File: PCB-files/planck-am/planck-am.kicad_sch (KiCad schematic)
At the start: 97 parts, among them U1 ProMicro

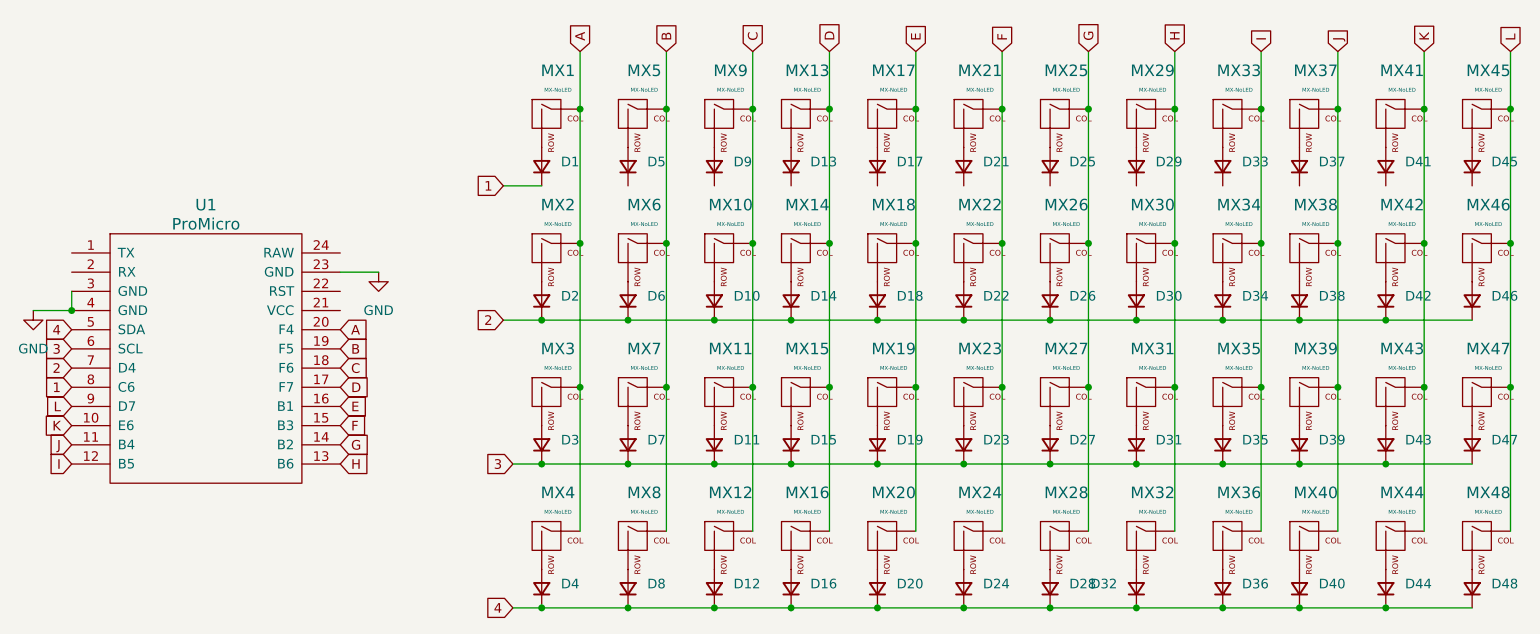
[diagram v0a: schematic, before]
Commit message: Commit
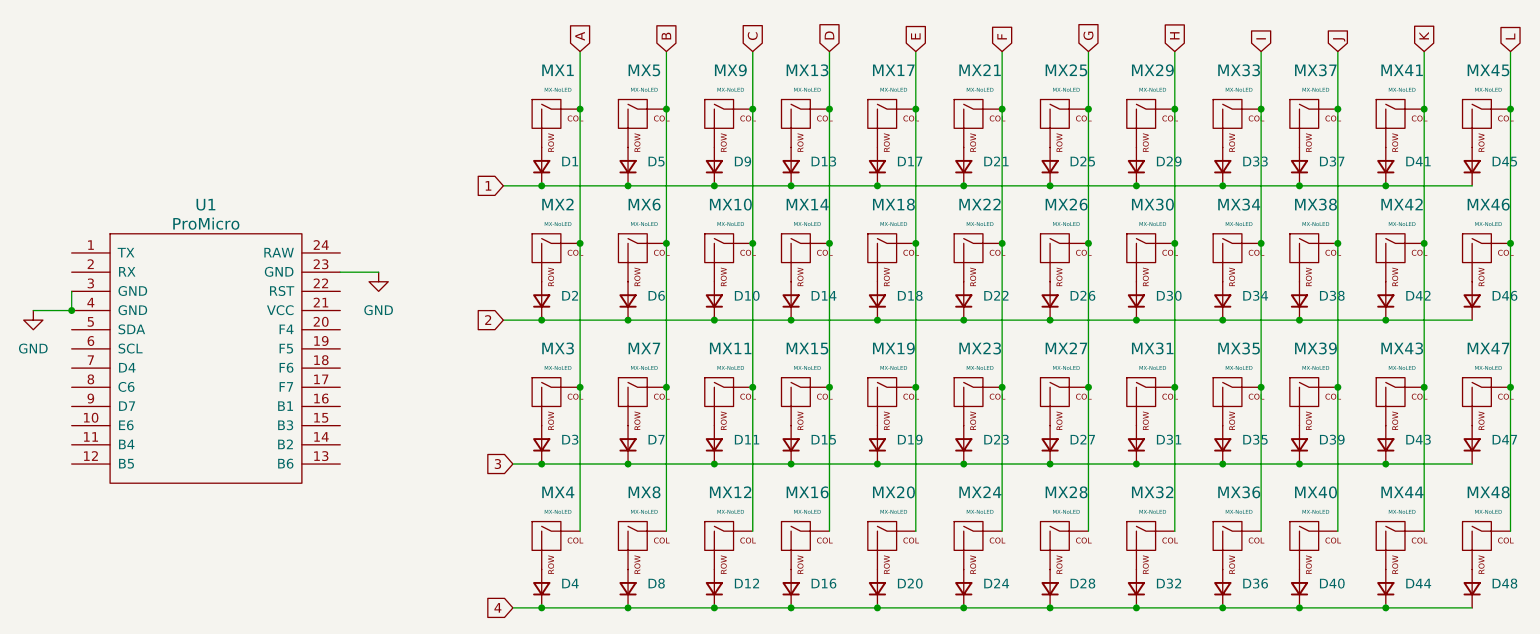
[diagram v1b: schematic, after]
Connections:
- net 1: now also D13.1 (K), D17.1 (K), D21.1 (K), D25.1 (K), D29.1 (K), D33.1 (K), D37.1 (K), D41.1 (K), D45.1 (K), D5.1 (K), D9.1 (K); no longer U1.8 (C6)
- net 2: no longer U1.7 (D4)
- net 3: no longer U1.6 (SCL)
- net 4: no longer U1.5 (SDA)
- net A: no longer U1.20 (F4)
- net B: no longer U1.19 (F5)
- net C: no longer U1.18 (F6)
- net D: no longer U1.17 (F7)
- net E: no longer U1.16 (B1)
- net F: no longer U1.15 (B3)
- net G: no longer U1.14 (B2)
- net H: no longer U1.13 (B6)
- net I: no longer U1.12 (B5)
- net J: no longer U1.11 (B4)
- net K: no longer U1.10 (E6)
- net L: no longer U1.9 (D7)
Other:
- moved on the sheet: D32

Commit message: grid is good, need to get vias
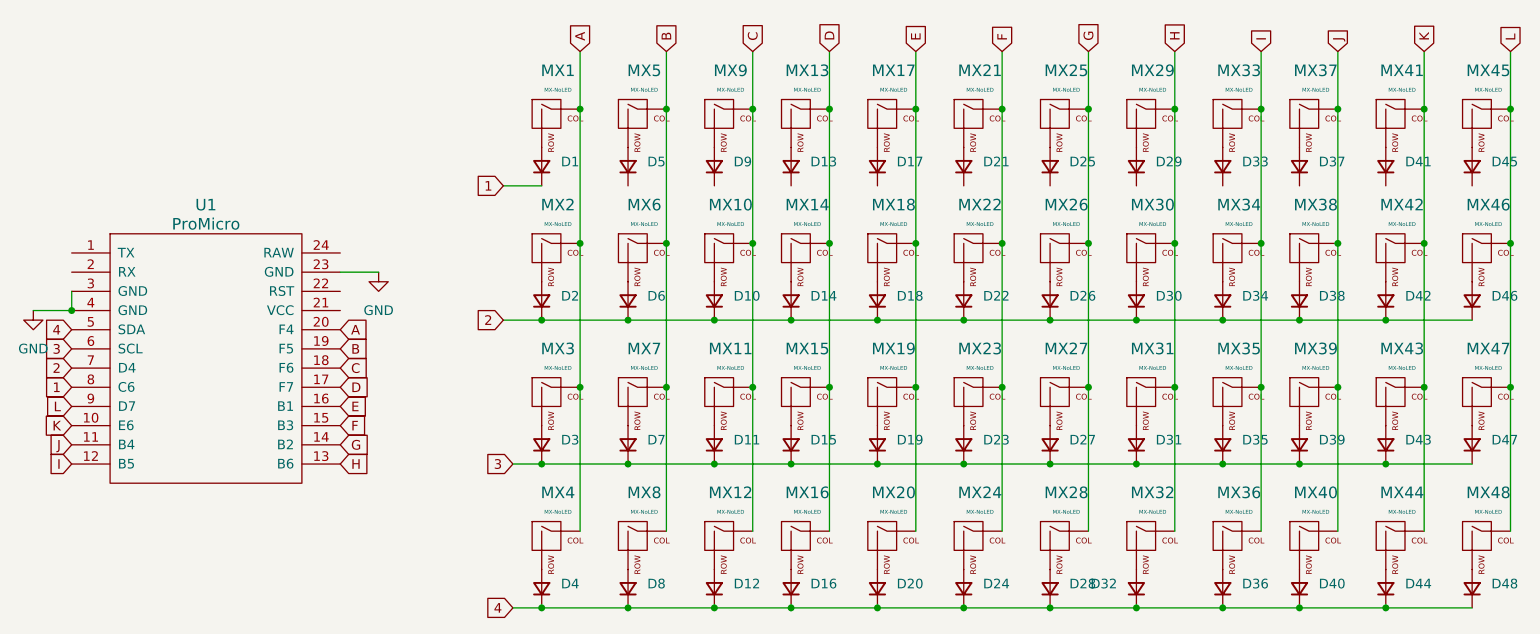
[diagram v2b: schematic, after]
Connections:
- net 1: now also U1.8 (C6); no longer D13.1 (K), D17.1 (K), D21.1 (K), D25.1 (K), D29.1 (K), D33.1 (K), D37.1 (K), D41.1 (K), D45.1 (K), D5.1 (K), D9.1 (K)
- net 2: now also U1.7 (D4)
- net 3: now also U1.6 (SCL)
- net 4: now also U1.5 (SDA)
- net A: now also U1.20 (F4)
- net B: now also U1.19 (F5)
- net C: now also U1.18 (F6)
- net D: now also U1.17 (F7)
- net E: now also U1.16 (B1)
- net F: now also U1.15 (B3)
- net G: now also U1.14 (B2)
- net H: now also U1.13 (B6)
- net I: now also U1.12 (B5)
- net J: now also U1.11 (B4)
- net K: now also U1.10 (E6)
- net L: now also U1.9 (D7)
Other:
- moved on the sheet: D32
